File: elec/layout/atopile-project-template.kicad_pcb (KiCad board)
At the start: 2 copper layers, 50.8 x 48.3 mm, 2 parts

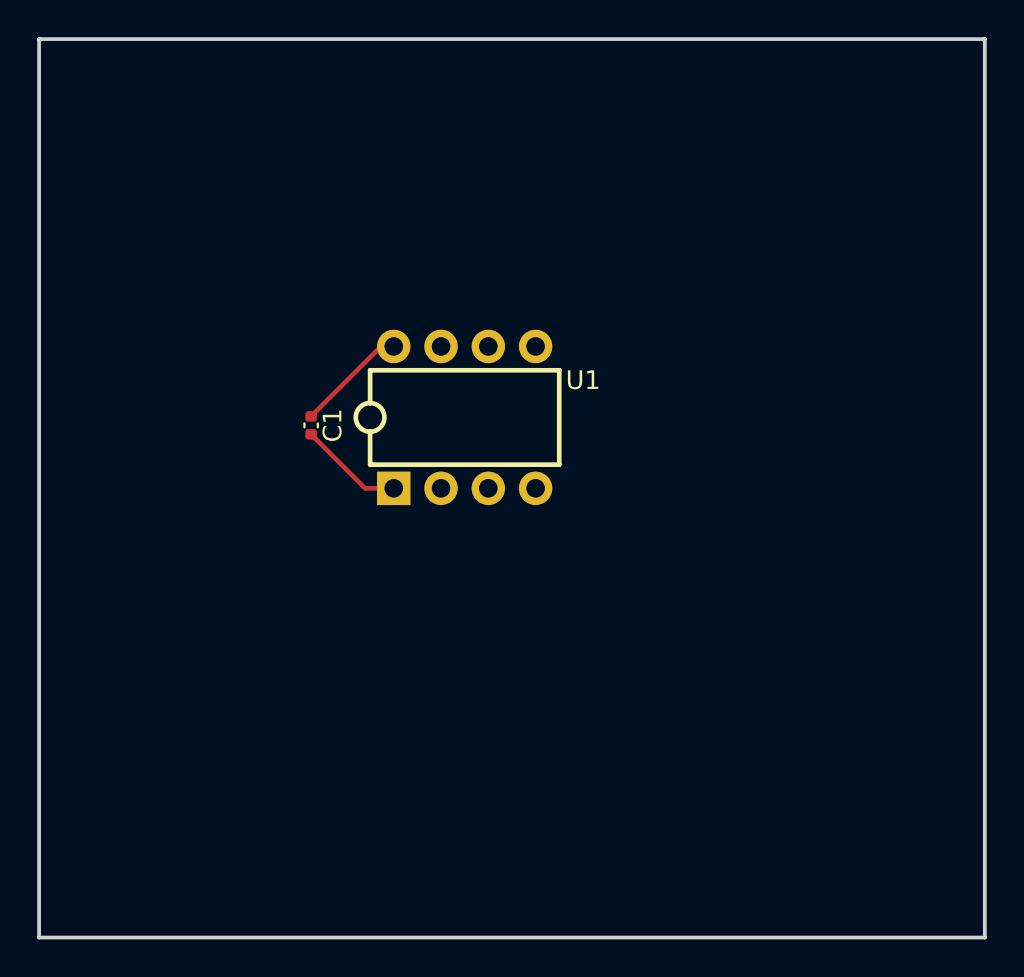
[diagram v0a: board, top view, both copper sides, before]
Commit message: add mech folder and git hash
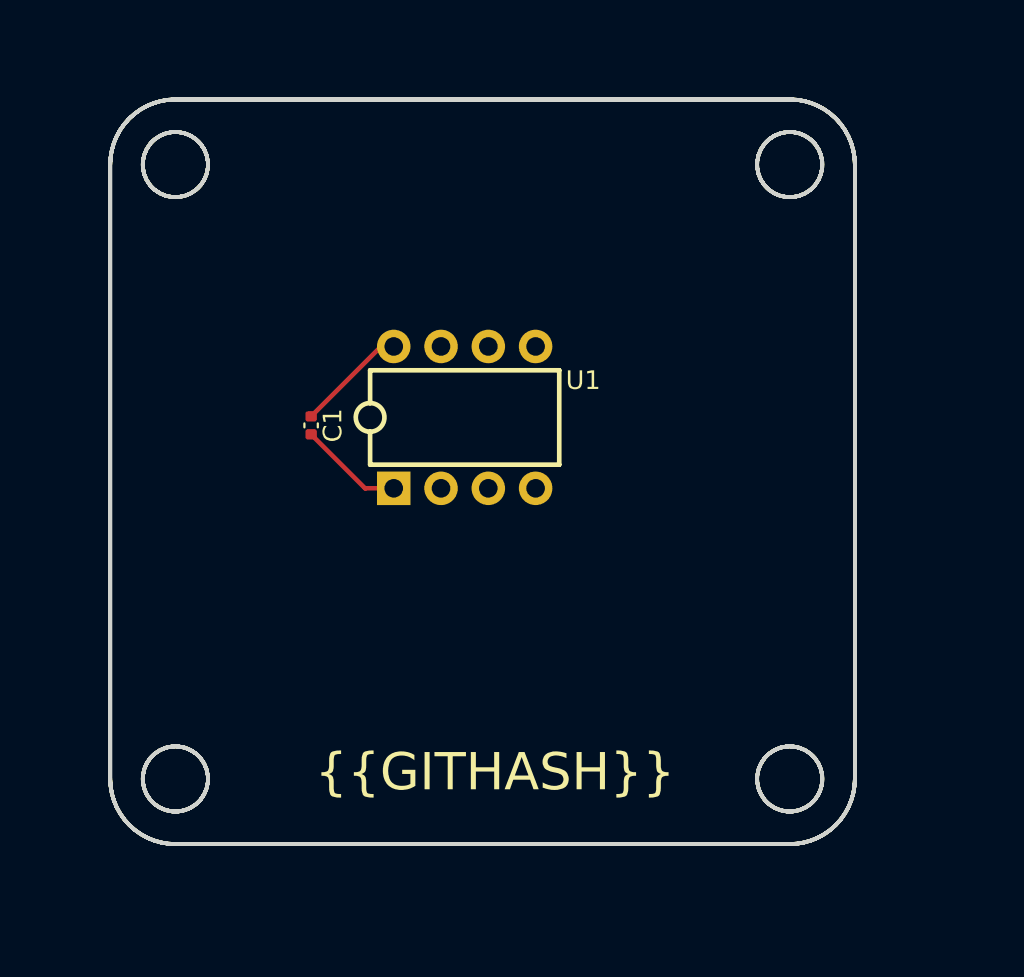
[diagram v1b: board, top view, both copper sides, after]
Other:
- board size 50.8 x 48.3 mm -> 40 x 40 mm
- board text added: "{{GITHASH}}"
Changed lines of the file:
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@@
     (fp_line (start 5.08 2.54) (end 5.08 -2.53)
       (stroke (width 0.25) (type solid)) (layer "F.SilkS"))
-    (fp_arc (start -5.093438 0.769883) (mid -5.073281 -0.769971) (end -5.08 0.77)
+    (fp_arc (start -5.093438 0.769883) (mid -5.073311 -0.769971) (end -5.08 0.77)
       (stroke (width 0.25) (type solid)) (layer "F.SilkS"))
     (fp_circle (center -3.94 4.45) (end -3.64 4.45)
@@
     )
   )
-  (gr_rect (start 119.38 73.66) (end 170.18 121.92)
-    (stroke (width 0.2) (type default)) (fill none) (layer "Edge.Cuts"))
+  (gr_line (start 123.2 113.4) (end 123.2 80.4)
+    (stroke (width 0.2) (type solid)) (layer "Edge.Cuts"))
+  (gr_arc (start 123.2 80.4) (mid 124.225126 77.925126) (end 126.7 76.9)
+    (stroke (width 0.2) (type solid)) (layer "Edge.Cuts"))
+  (gr_circle (center 159.7 80.4) (end 161.45 80.4)
+    (stroke (width 0.2) (type solid)) (fill none) (layer "Edge.Cuts"))
+  (gr_arc (start 159.7 76.9) (mid 162.174874 77.925126) (end 163.2 80.4)
+    (stroke (width 0.2) (type solid)) (layer "Edge.Cuts"))
+  (gr_line (start 163.2 113.4) (end 163.2 80.4)
+    (stroke (width 0.2) (type solid)) (layer "Edge.Cuts"))
+  (gr_arc (start 163.2 113.4) (mid 162.174874 115.874874) (end 159.7 116.9)
+    (stroke (width 0.2) (type solid)) (layer "Edge.Cuts"))
+  (gr_line (start 159.7 116.9) (end 126.7 116.9)
+    (stroke (width 0.2) (type solid)) (layer "Edge.Cuts"))
+  (gr_arc (start 159.7 76.9) (mid 162.174874 77.925126) (end 163.2 80.4)
+    (stroke (width 0.2) (type solid)) (layer "Edge.Cuts"))
+  (gr_arc (start 159.7 76.9) (mid 162.174874 77.925126) (end 163.2 80.4)
+    (stroke (width 0.2) (type solid)) (layer "Edge.Cuts"))
+  (gr_circle (center 126.7 113.4) (end 128.45 113.4)
+    (stroke (width 0.2) (type solid)) (fill none) (layer "Edge.Cuts"))
+  (gr_arc (start 163.2 113.4) (mid 162.174874 115.874874) (end 159.7 116.9)
+    (stroke (width 0.2) (type solid)) (layer "Edge.Cuts"))
+  (gr_arc (start 123.2 80.4) (mid 124.225126 77.925126) (end 126.7 76.9)
+    (stroke (width 0.2) (type solid)) (layer "Edge.Cuts"))
+  (gr_line (start 126.7 76.9) (end 159.7 76.9)
+    (stroke (width 0.2) (type solid)) (layer "Edge.Cuts"))
+  (gr_arc (start 126.7 116.9) (mid 124.225126 115.874874) (end 123.2 113.4)
+    (stroke (width 0.2) (type solid)) (layer "Edge.Cuts"))
+  (gr_line (start 163.2 80.4) (end 163.2 113.4)
+    (stroke (width 0.2) (type solid)) (layer "Edge.Cuts"))
+  (gr_arc (start 163.2 113.4) (mid 162.174874 115.874874) (end 159.7 116.9)
+    (stroke (width 0.2) (type solid)) (layer "Edge.Cuts"))
+  (gr_circle (center 159.7 113.4) (end 161.45 113.4)
+    (stroke (width 0.2) (type solid)) (fill none) (layer "Edge.Cuts"))
+  (gr_circle (center 126.7 80.4) (end 128.45 80.4)
+    (stroke (width 0.2) (type solid)) (fill none) (layer "Edge.Cuts"))
+  (gr_line (start 163.2 80.4) (end 163.2 113.4)
+    (stroke (width 0.2) (type solid)) (layer "Edge.Cuts"))
+  (gr_arc (start 126.7 116.9) (mid 124.225126 115.874874) (end 123.2 113.4)
+    (stroke (width 0.2) (type solid)) (layer "Edge.Cuts"))
+  (gr_circle (center 126.7 113.4) (end 128.45 113.4)
+    (stroke (width 0.2) (type solid)) (fill none) (layer "Edge.Cuts"))
+  (gr_circle (center 126.7 80.4) (end 128.45 80.4)
+    (stroke (width 0.2) (type solid)) (fill none) (layer "Edge.Cuts"))
+  (gr_circle (center 159.7 113.4) (end 161.45 113.4)
+    (stroke (width 0.2) (type solid)) (fill none) (layer "Edge.Cuts"))
+  (gr_arc (start 159.7 76.9) (mid 162.174874 77.925126) (end 163.2 80.4)
+    (stroke (width 0.2) (type solid)) (layer "Edge.Cuts"))
+  (gr_line (start 126.7 76.9) (end 159.7 76.9)
+    (stroke (width 0.2) (type solid)) (layer "Edge.Cuts"))
+  (gr_line (start 123.2 80.4) (end 123.2 113.4)
+    (stroke (width 0.2) (type solid)) (layer "Edge.Cuts"))
+  (gr_circle (center 126.7 113.4) (end 128.45 113.4)
+    (stroke (width 0.2) (type solid)) (fill none) (layer "Edge.Cuts"))
+  (gr_line (start 163.2 113.4) (end 163.2 80.4)
+    (stroke (width 0.2) (type solid)) (layer "Edge.Cuts"))
+  (gr_circle (center 126.7 80.4) (end 128.45 80.4)
+    (stroke (width 0.2) (type solid)) (fill none) (layer "Edge.Cuts"))
+  (gr_circle (center 159.7 113.4) (end 161.45 113.4)
+    (stroke (width 0.2) (type solid)) (fill none) (layer "Edge.Cuts"))
+  (gr_circle (center 126.7 80.4) (end 128.45 80.4)
+    (stroke (width 0.2) (type solid)) (fill none) (layer "Edge.Cuts"))
+  (gr_circle (center 126.7 113.4) (end 128.45 113.4)
+    (stroke (width 0.2) (type solid)) (fill none) (layer "Edge.Cuts"))
+  (gr_arc (start 126.7 116.9) (mid 124.225126 115.874874) (end 123.2 113.4)
+    (stroke (width 0.2) (type solid)) (layer "Edge.Cuts"))
+  (gr_line (start 123.2 80.4) (end 123.2 113.4)
+    (stroke (width 0.2) (type solid)) (layer "Edge.Cuts"))
+  (gr_circle (center 159.7 113.4) (end 161.45 113.4)
+    (stroke (width 0.2) (type solid)) (fill none) (layer "Edge.Cuts"))
+  (gr_arc (start 123.2 80.4) (mid 124.225126 77.925126) (end 126.7 76.9)
+    (stroke (width 0.2) (type solid)) (layer "Edge.Cuts"))
+  (gr_arc (start 163.2 113.4) (mid 162.174874 115.874874) (end 159.7 116.9)
+    (stroke (width 0.2) (type solid)) (layer "Edge.Cuts"))
+  (gr_line (start 159.7 116.9) (end 126.7 116.9)
+    (stroke (width 0.2) (type solid)) (layer "Edge.Cuts"))
+  (gr_line (start 126.7 116.9) (end 159.7 116.9)
+    (stroke (width 0.2) (type solid)) (layer "Edge.Cuts"))
+  (gr_line (start 126.7 116.9) (end 159.7 116.9)
+    (stroke (width 0.2) (type solid)) (layer "Edge.Cuts"))
+  (gr_circle (center 159.7 80.4) (end 161.45 80.4)
+    (stroke (width 0.2) (type solid)) (fill none) (layer "Edge.Cuts"))
+  (gr_arc (start 123.2 80.4) (mid 124.225126 77.925126) (end 126.7 76.9)
+    (stroke (width 0.2) (type solid)) (layer "Edge.Cuts"))
+  (gr_circle (center 159.7 80.4) (end 161.45 80.4)
+    (stroke (width 0.2) (type solid)) (fill none) (layer "Edge.Cuts"))
+  (gr_line (start 126.7 76.9) (end 159.7 76.9)
+    (stroke (width 0.2) (type solid)) (layer "Edge.Cuts"))
+  (gr_line (start 123.2 113.4) (end 123.2 80.4)
+    (stroke (width 0.2) (type solid)) (layer "Edge.Cuts"))
+  (gr_arc (start 126.7 116.9) (mid 124.225126 115.874874) (end 123.2 113.4)
+    (stroke (width 0.2) (type solid)) (layer "Edge.Cuts"))
+  (gr_line (start 126.7 76.9) (end 159.7 76.9)
+    (stroke (width 0.2) (type solid)) (layer "Edge.Cuts"))
+  (gr_circle (center 159.7 80.4) (end 161.45 80.4)
+    (stroke (width 0.2) (type solid)) (fill none) (layer "Edge.Cuts"))
+  (gr_text "{{GITHASH}} " (at 134.2 114.2) (layer "F.SilkS")
+    (effects (font (size 2 2) (thickness 0.1)) (justify left bottom))
+  )
   (segment (start 137.744156 90.17) (end 133.991711 93.922445) (width 0.25) (layer "F.Cu") (net 1))
   (segment (start 133.991711 93.922445) (end 133.991711 93.930054) (width 0.25) (layer "F.Cu") (net 1))
@@
   (segment (start 136.891657 97.79) (end 133.991711 94.890054) (width 0.25) (layer "F.Cu") (net 2))
   (segment (start 138.43 97.79) (end 136.891657 97.79) (width 0.25) (layer "F.Cu") (net 2))
+  (group "" (id 4e3ea3a3-d408-4ad8-873b-ebd87bd265e7)
+    (members
+      00e9e413-fe55-4320-b973-81fdf0b4cc24
+      0fc59361-2a09-4339-8464-495b51280d7e
+      12fa702a-45c0-4228-8798-0b1dff755467
+      1492c265-9600-4fac-807f-5aa558c04698
+      198da371-5ea4-4cce-89c6-a85e4e6fd5a2
+      20f5aec2-f82f-440a-88e0-7c770baed97c
+      23a80093-b831-494f-9bba-68421986c52c
+      26636bbf-1c2a-4df7-88c1-c20fa037cc7a
+      2b89afd7-dd24-41f4-85c0-9b0b291f5c57
+      2fc81b31-9add-483d-8263-1bf15a86faaf
+      34b8980e-5130-409d-83b7-73880c0817a4
+      36ab1010-5541-4b38-b363-4a27707f3202
+      3788308b-797f-4a53-8c52-00e61ef351dc
+      3a9095b0-7e4b-4c7f-aacb-bc9d3781fe0b
+      3d3db7c2-c89f-4be3-8e91-39fe7a9cebf3
+      3fee8cd8-9e80-4a1a-bcb8-484494266562
+      41a35e0c-0cd9-4884-83bf-a5f765917301
+      4354ef4b-af71-4b02-9a7b-930427945da3
+      4651f4aa-f85a-4992-9560-eff928a0e15f
+      4accd462-b544-44a7-ac19-ab4f0dd67dcb
+      4c413f87-443c-40db-810d-24d0127db4d1
+      55d6076c-5015-49df-810a-c55f5388576e
+      65b328d4-d955-42de-9ccd-564ff2e6e4da
+      65dc38af-d159-41f4-ba48-e112a9d8b717
+      69dabe7c-0c06-4af2-9c4e-d415cbc6d866
+      73c11e5d-a507-4a2f-8e42-2453482f9ba0
+      7609faaa-2ca7-4089-85bb-2ec6ff9f31bd
+      7dc85215-0547-4a98-92f9-7acc82968b0d
+      807b6513-e212-46b2-b774-80b1d14145d6
+      8278bfc6-c86b-4bbe-bee5-200ba347b53f
+      8adfd382-b7b3-40dc-abbc-698204ed259d
+      8d118edb-2a69-4839-a0e0-808db2b83267
+      9668049e-ace8-48bb-aaac-8c53c3bb8f64
+      abd0a840-cb12-4cfc-a11d-66180da66a73
+      ad767e51-32fc-4ffe-95cc-17d42beb101f
+      af147bb3-b7ba-4977-ab61-3eda152bc58e
+      b39eb833-0b6b-454c-91fa-8515f3b4c5a4
+      ba81428c-9237-4b33-8a8a-b0ef2c7129aa
+      bdb82cab-935c-4872-93ce-aa33a6ca8e3e
+      c200e945-b1eb-4ba9-846c-549b5888c1c9
+      c85d377d-8655-43a5-93e8-60ea0121da42
+      cdd996d3-1fa6-4070-aa95-b92a7005f8a0
+      db81513a-caef-41e6-97f5-8d6aa049d4d7
+      dbcff90b-bfca-4e87-8d37-d1133e183e20
+      e3c8b72a-7566-4951-ab61-af945b777583
+      e8b9d802-86fd-4393-87e2-6b6d02952d22
+      ec90ed93-4ada-407b-9626-0f35de0bac02
+      eeb07992-fe8e-4cf4-bf6c-0cf18fd77681
+    )
+  )
 )
